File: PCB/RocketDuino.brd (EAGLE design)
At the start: 73 x 41 mm, 41 parts, among them J1 FTDI, Y1 16MHZ

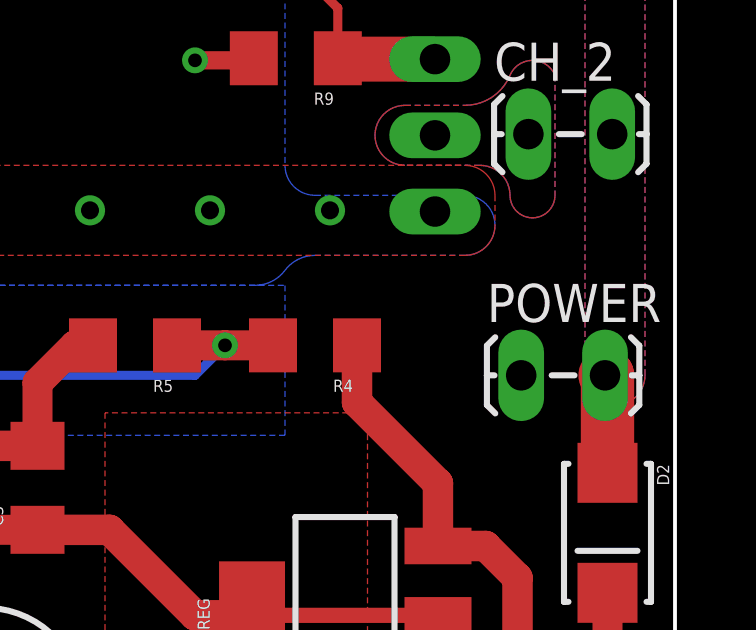
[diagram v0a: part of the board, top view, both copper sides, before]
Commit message: Very minor board movements
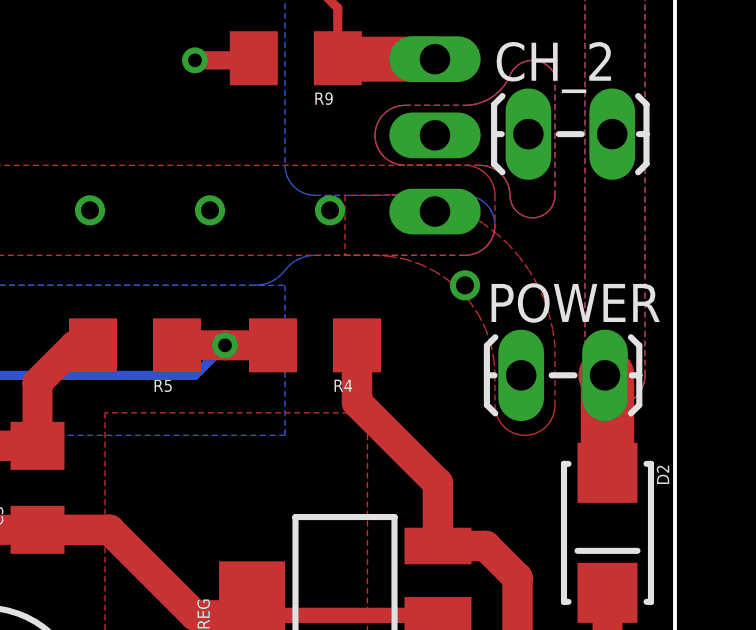
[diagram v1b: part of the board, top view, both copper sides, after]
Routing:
- net GND: vias 20 -> 21
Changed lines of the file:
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@@
 <wire x1="45.75" y1="13.75" x2="45.85" y2="13.65" width="1.016" layer="1"/>
 <wire x1="45.85" y1="13.65" x2="48" y2="13.65" width="1.016" layer="1"/>
+<polygon width="0.254" layer="1" isolate="1" thermals="no" rank="4">
+<vertex x="62" y="20"/>
+<vertex x="63" y="20" curve="-90"/>
+<vertex x="67" y="16"/>
+<vertex x="67" y="15" curve="90"/>
+<vertex x="68" y="14" curve="90"/>
+<vertex x="69" y="15"/>
+<vertex x="69" y="17" curve="90"/>
+<vertex x="63" y="22"/>
+<vertex x="62" y="22"/>
+</polygon>
+<via x="66" y="19" extent="1-16" drill="0.6"/>
 </signal>
 <signal name="RESET">
